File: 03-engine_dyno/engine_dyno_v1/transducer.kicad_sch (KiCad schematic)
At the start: 6 parts, among them J2 Screw_Terminal_01x05, U6 INA827AIDGKR, U7 AD630ARZ, U8 OPA192IDBVR, U9 ADS1120IPWR

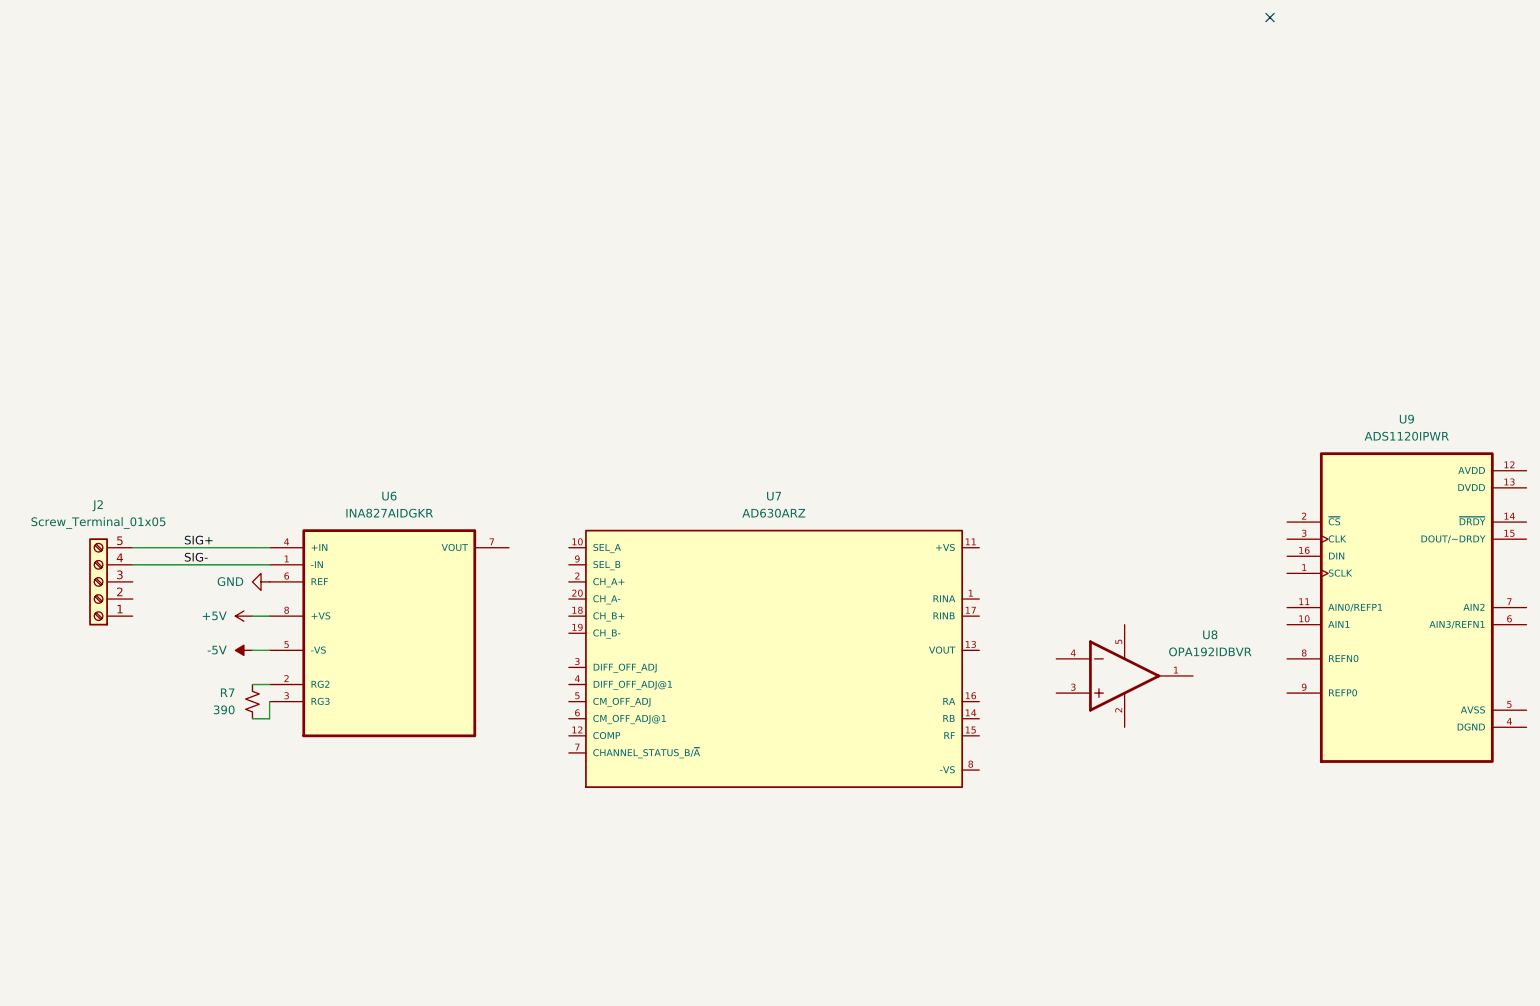
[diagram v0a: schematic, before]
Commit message: transducer and hall preliminary design
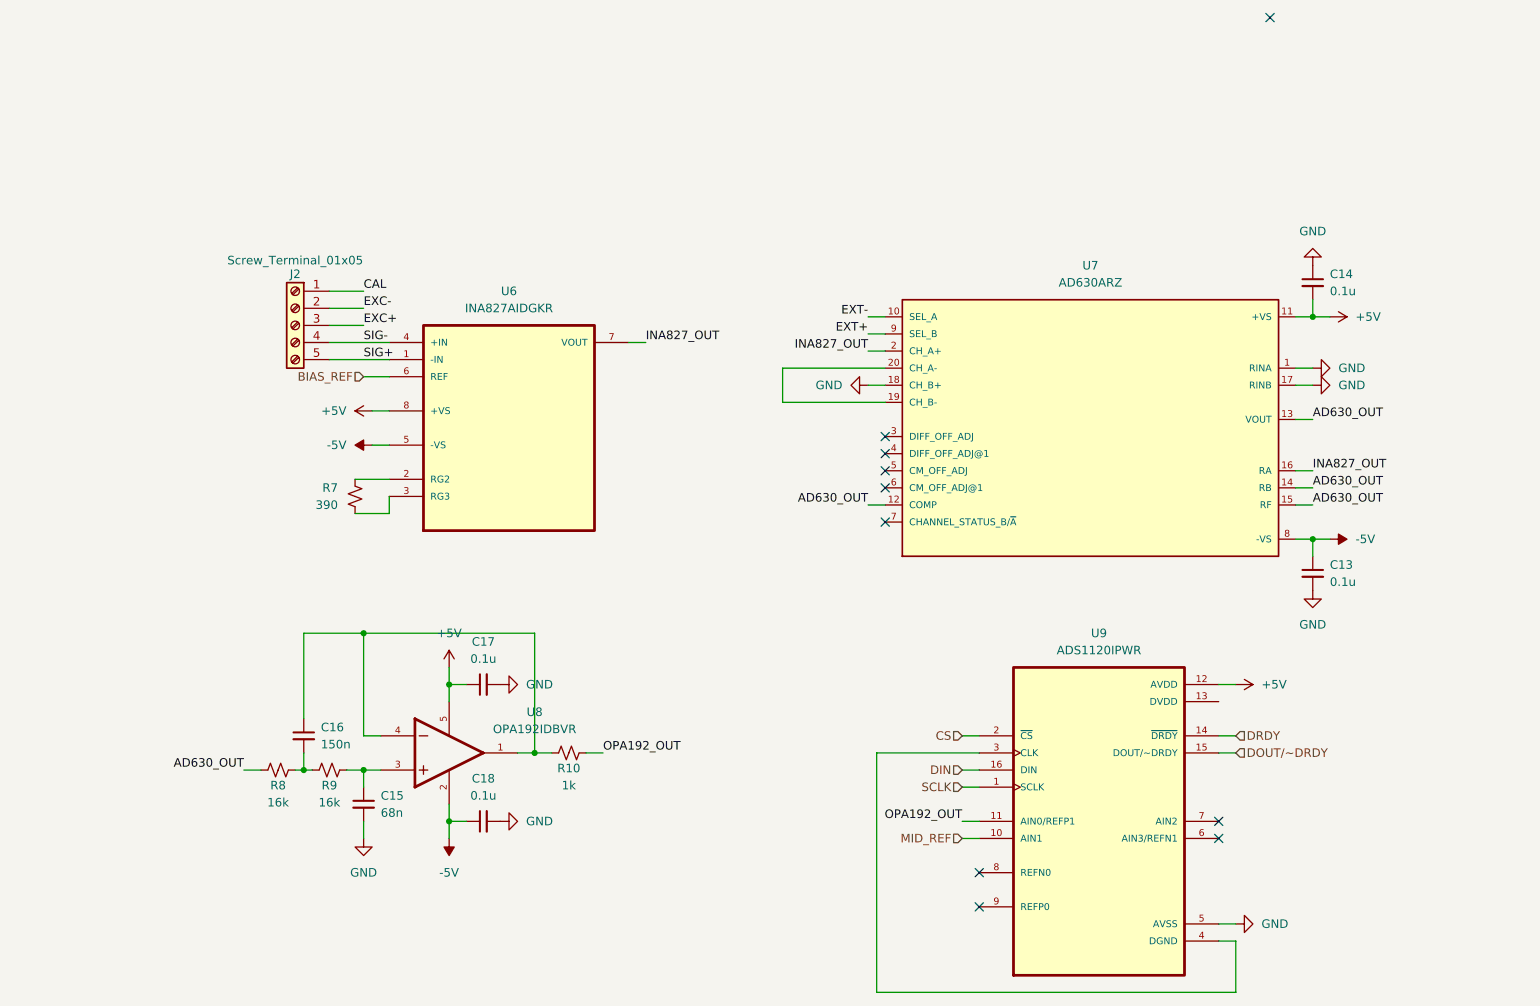
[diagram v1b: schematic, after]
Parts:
- added C13, C14, C17, C18: 0.1u, symbol Device:C_Small
- added C15: 68n, symbol Device:C_Small
- added C16: 150n, symbol Device:C_Small
- added R10: 1k, symbol Device:R_Small_US
- added R8, R9: 16k, symbol Device:R_Small_US
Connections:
- net +5V: now also U7.11 (+VS), U8.5, U9.12 (AVDD), C14.2, C17.1
- net -5V: now also U7.8 (-VS), U8.2, C13.1, C18.1
- net GND: now also U7.1 (RINA), U7.17 (RINB), U7.18 (CH_B+), U9.5 (AVSS), C13.2, C14.1, C15.2, C17.2, C18.2; no longer U6.6 (REF)
- net SIG+: now also U6.1 (-IN); no longer U6.4 (+IN)
- net SIG-: now also U6.4 (+IN); no longer U6.1 (-IN)
- net CAL: now reaches J2.1 (Pin_1)
- net EXC-: now reaches J2.2 (Pin_2)
- net EXC+: now reaches J2.3 (Pin_3)
- net at U8.1: now also U8.4, C16.1, R10.1
- net at U8.3: now also C15.1, R9.2
- net INA827_OUT: now reaches U6.7 (VOUT)
- net INA827_OUT: now also U7.16 (RA), U7.2 (CH_A+)
- net SCLK: now reaches U9.1 (SCLK)
- net MID_REF: now reaches U9.10 (AIN1)
- net OPA192_OUT: now reaches U9.11 (AIN0/REFP1)
- net OPA192_OUT: now also R10.2
- net DRDY: now reaches U9.14 (~{DRDY})
- net DOUT/~DRDY: now reaches U9.15 (DOUT/~DRDY)
- net DIN: now reaches U9.16 (DIN)
- net CS: now reaches U9.2 (~{CS})
- net at U9.3 (CLK): now also U9.4 (DGND)
- net EXT-: now reaches U7.10 (SEL_A)
- net AD630_OUT: now reaches U7.12 (COMP)
- net AD630_OUT: now also U7.13 (VOUT), U7.14 (RB), U7.15 (RF), R8.1
- net at U7.19 (CH_B-): now also U7.20 (CH_A-)
- net EXT+: now reaches U7.9 (SEL_B)
- new net: C16.2, R8.2, R9.1
- new net BIAS_REF: U6.6 (REF)
- no-connect marks 1 -> 10
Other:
- moved on the sheet: J2, R7, U6, U7, U8, U9
